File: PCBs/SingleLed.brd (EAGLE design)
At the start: 15 x 28.7 mm, 4 parts

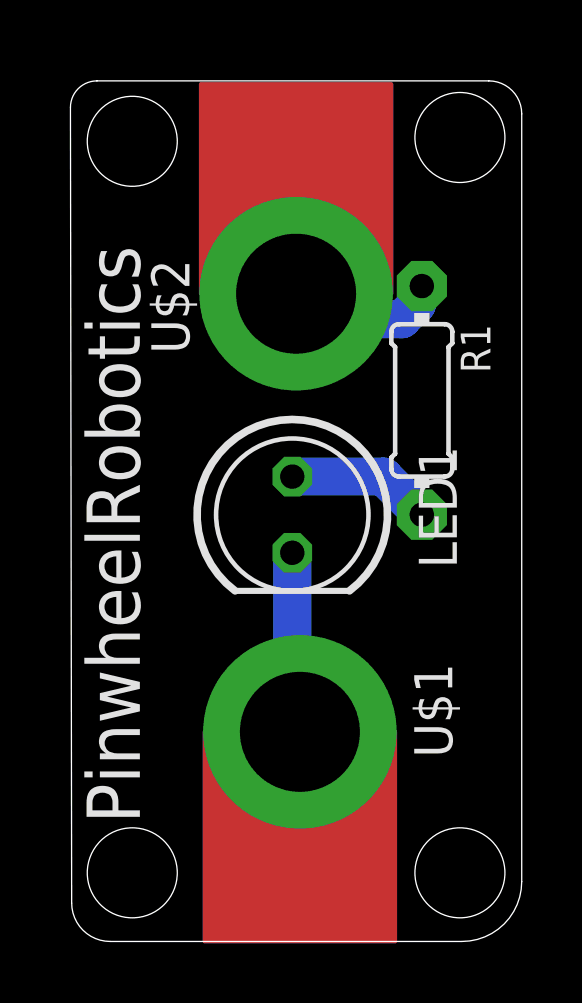
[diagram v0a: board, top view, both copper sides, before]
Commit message: New Update
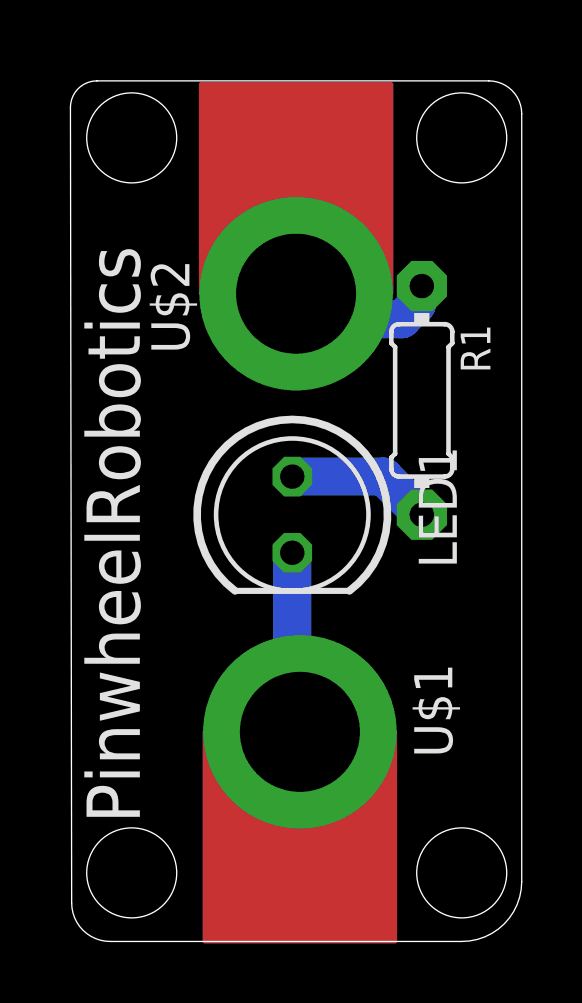
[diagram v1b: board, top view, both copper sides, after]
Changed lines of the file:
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@@
 <drawing>
 <settings>
-<setting alwaysvectorfont="yes"/>
+<setting alwaysvectorfont="no"/>
 <setting verticaltext="up"/>
 </settings>
@@
 <wire x1="28.902534375" y1="42.4" x2="15.84123125" y2="42.4" width="0" layer="20"/>
 <wire x1="15.84123125" y1="42.4" x2="14.95735625" y2="41.5157875" width="0" layer="20" curve="90.021878"/>
-<hole x="17.018" y="40.386" drill="3"/>
-<hole x="17.018" y="16.002" drill="3"/>
-<hole x="27.94" y="16.002" drill="3"/>
-<hole x="27.94" y="40.513" drill="3"/>
+<hole x="17" y="40.5" drill="3"/>
+<hole x="17" y="16" drill="3"/>
+<hole x="28" y="16" drill="3"/>
+<hole x="28" y="40.5" drill="3"/>
 <text x="17.272" y="17.653" size="1.778" layer="21" rot="R90">PinwheelRobotics</text>
 <text x="29.718" y="37.465" size="1.778" layer="22" rot="MR270">care@pinwheel.in</text>
